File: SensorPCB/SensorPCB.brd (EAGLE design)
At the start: 37 x 65 mm, 32 parts, among them T1 33u

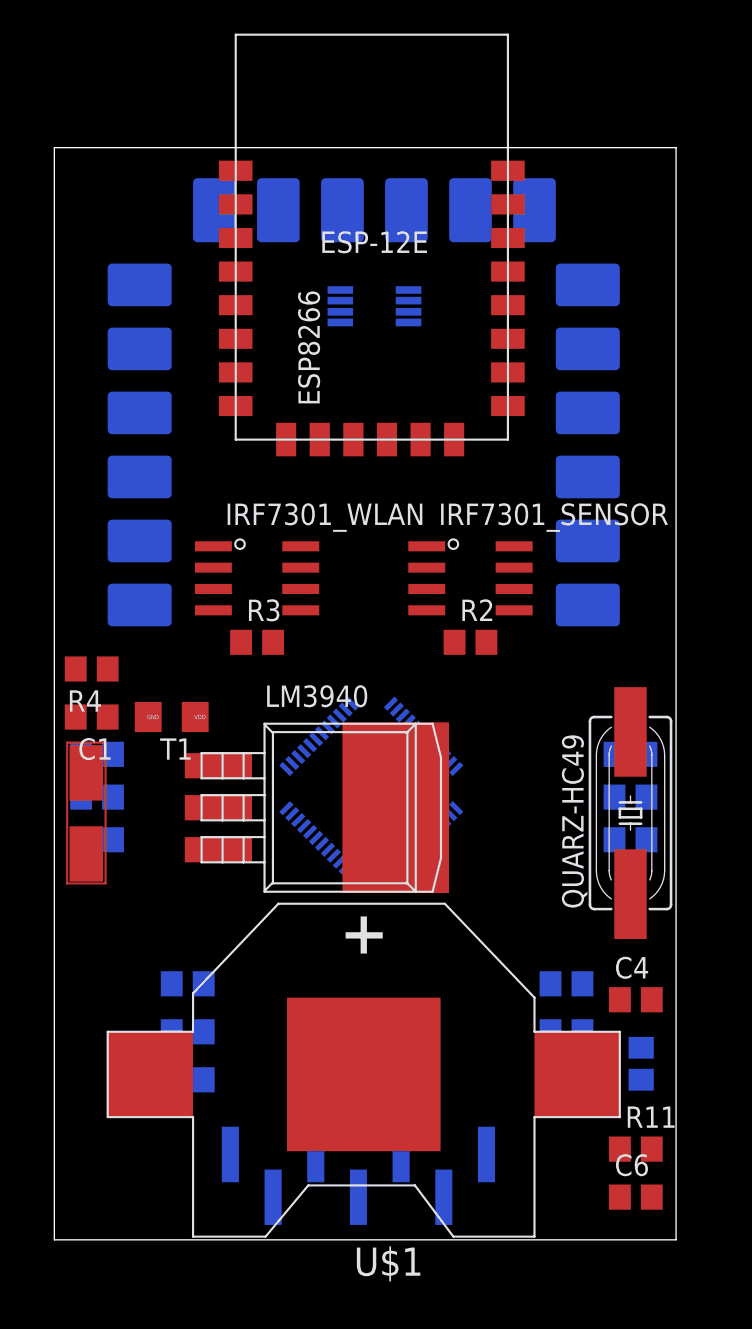
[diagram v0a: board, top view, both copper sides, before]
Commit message: routing
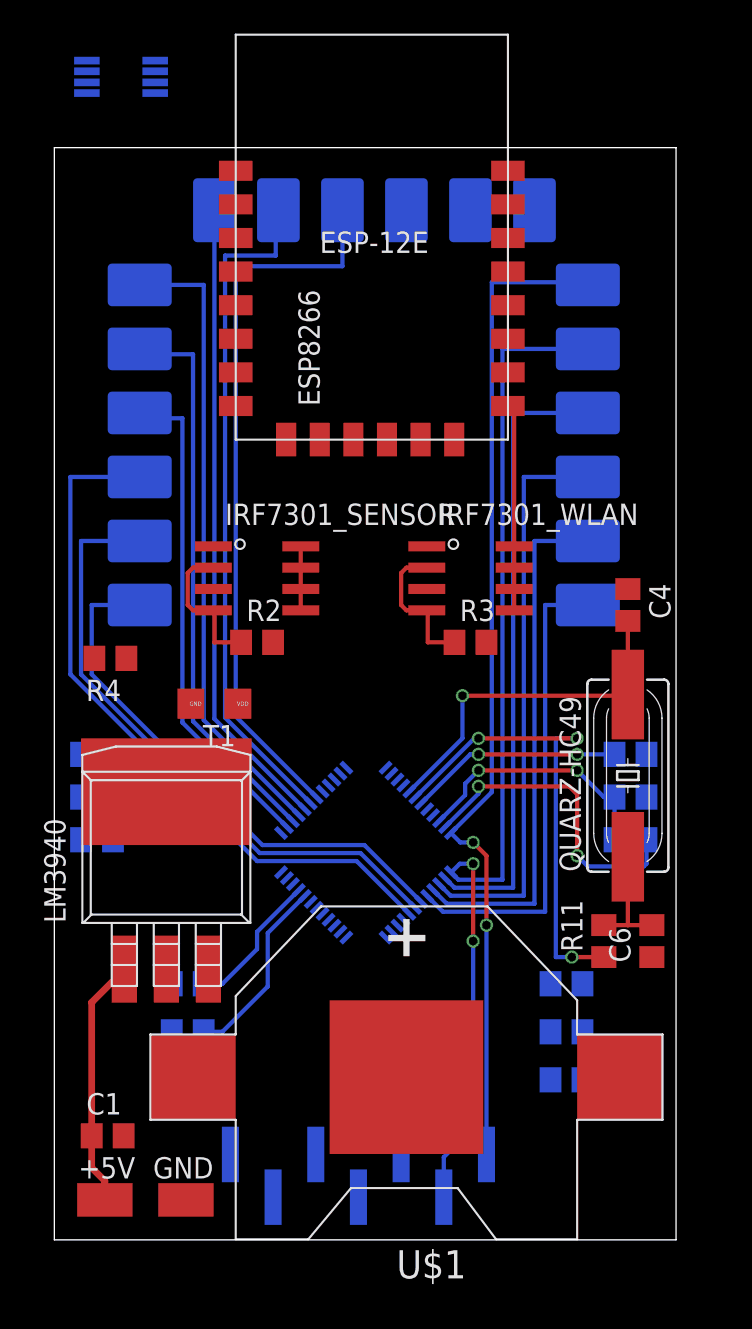
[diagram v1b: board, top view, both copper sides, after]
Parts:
- moved C1 24.9 mm to (3.17, 6.19), turned to 0 degrees
- moved C4 23.5 mm to (34.1, 37.8), turned to 270 degrees
- moved U$2 23.3 mm to (5.40, 2.38), turned to 180 degrees
- moved MCP9808 20.3 mm to (3.97, 69.2)
- moved C6 15.3 mm to (35.6, 17.8), turned to 90 degrees
- moved IRF7301_SENSOR 12.7 mm to (12.1, 39.4)
- moved IRF7301_WLAN 12.7 mm to (24.8, 39.4)
- moved R2 12.7 mm to (12.1, 35.6)
- moved R3 12.7 mm to (24.8, 35.6)
- moved R11 12.5 mm to (32.7, 17.8), turned to 90 degrees
- moved LM3940 11.2 mm to (6.67, 24.1), turned to 0 degrees
- moved STM32L051C8T6 3.82 mm to (18.5, 23.0)
- moved T1 2.66 mm to (9.53, 31.9)
- moved U$1 2.54 mm to (21.0, 9.68)
- moved QUARZ-HC49 2.23 mm to (34.1, 27.6)
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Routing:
- net USART2_RX_SENSOR: track 0.00 -> 62.0 mm, vias 0 -> 2
- net USART2_TX_SENSOR: track 0.00 -> 60.0 mm, vias 0 -> 2
- net I2C1_SDA_SENSOR: track 0.00 -> 43.3 mm
- net PB2: track 0.00 -> 42.0 mm
- net I2C1_SCL_SENSOR: track 0.00 -> 40.5 mm
- net SPI1_MOSI_SENSOR: track 0.00 -> 37.9 mm
- net SPI1_MISO_SENSOR: track 0.00 -> 37.7 mm
- net PB1: track 0.00 -> 37.1 mm
- net PA4: track 0.00 -> 37.0 mm
- net PA5: track 0.00 -> 34.1 mm
- net SPI1_SCK_SENSOR: track 0.00 -> 33.6 mm
- net PB0: track 0.00 -> 32.2 mm
- net PA6: track 0.00 -> 31.1 mm
- net SPI1_NSS_SENSOR: track 0.00 -> 29.6 mm
- net OSC_OUT: track 0.00 -> 28.5 mm, vias 0 -> 3
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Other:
- board text added: "+5V"
- board text added: "GND"
